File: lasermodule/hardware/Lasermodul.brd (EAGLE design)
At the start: 89 parts, among them IC1 MEGA8-AI

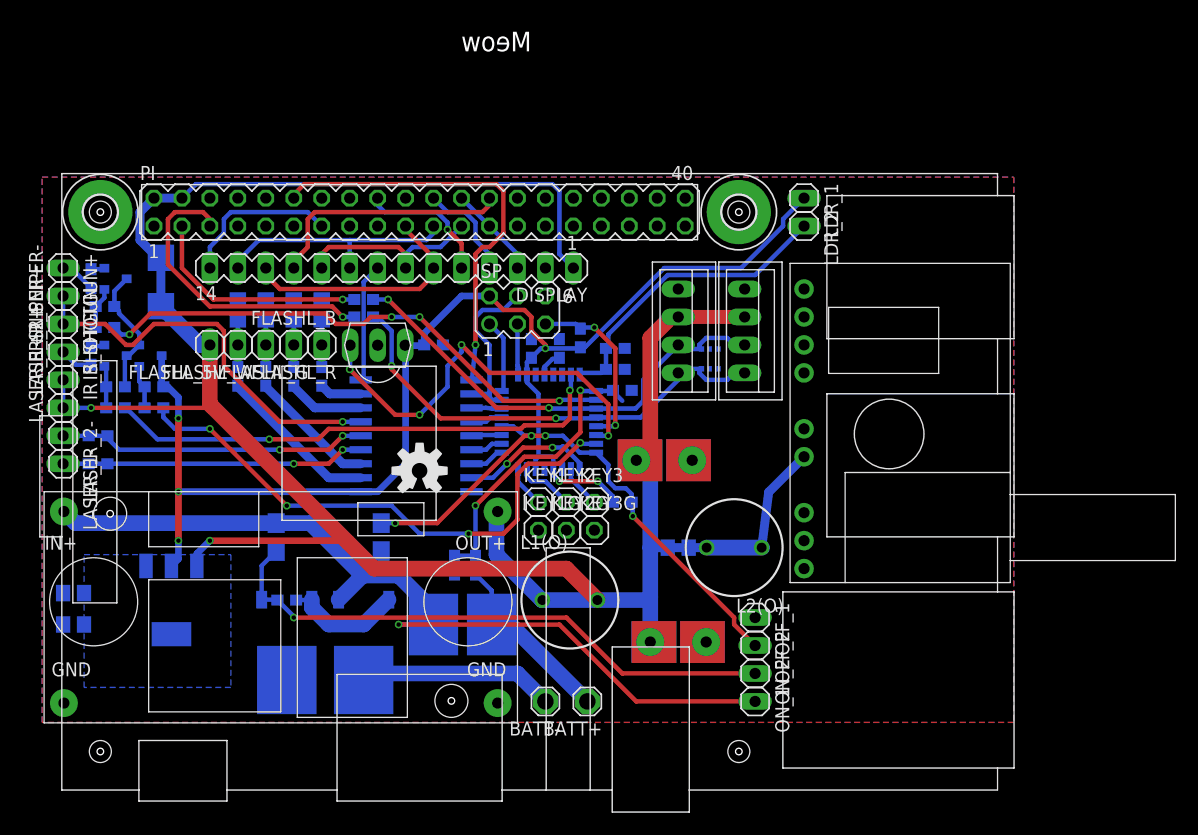
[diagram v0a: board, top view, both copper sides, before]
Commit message: routing
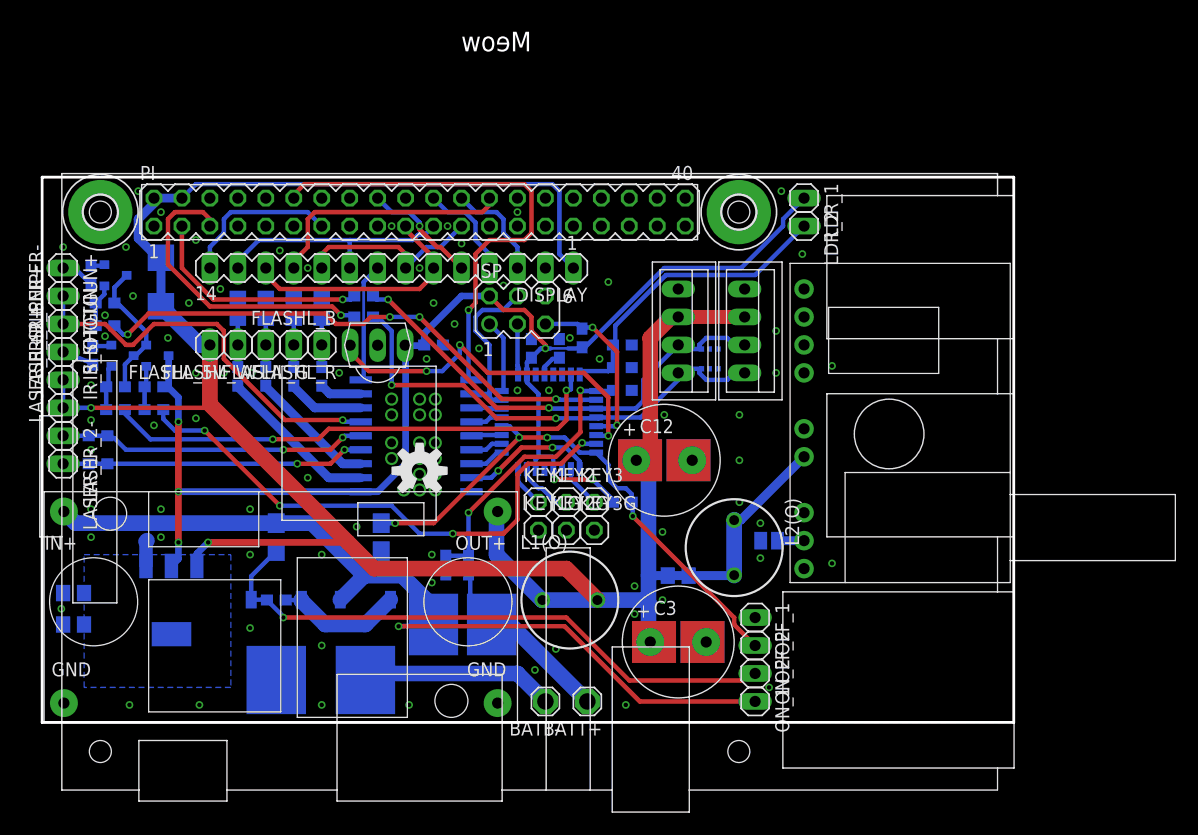
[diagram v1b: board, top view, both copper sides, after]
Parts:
- added SJ1: (no value), jumper:SJ
- moved R3(O) 2.54 mm to (57.8, 13.3)
- moved ON 0.95 mm to (21.3, 6.35)
- moved R9 0.95 mm to (21.3, 11.1)
- moved R5 0.79 mm to (36.7, 14.3)
- moved R16 0.71 mm to (52.7, 34.3)
- moved C4 0.65 mm to (52.7, 32.2)
- moved P-FET1 0.63 mm to (10.5, 33.3)
- moved P-FET2 0.63 mm to (7.30, 33.3)
- moved R4 0.63 mm to (38.7, 14.3)
- moved P-FET3 0.32 mm to (6.67, 40.6)
- moved R23 0.32 mm to (5.71, 38.1)
- moved R24 0.32 mm to (4.45, 40.6)
- moved R6 0.32 mm to (29.2, 38.7)
- moved R22 0.16 mm to (5.71, 36.0)
- moved R21 0.16 mm to (4.60, 33.3)
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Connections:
- net +5V: now also C12.+, C3.+; no longer C12.+A, C12.+B, C12.+C, C3.+A, C3.+B, C3.+C
- net AMP_IN_AGND: now also SJ1.2
- net GND: now also C12.-, C3.-, SJ1.1; no longer C12.-A, C12.-B, C12.-C, C3.-A, C3.-B, C3.-C
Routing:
- net I_BACKLIGHT: track 38.6 -> 44.1 mm
- net RX: track 37.7 -> 32.9 mm, vias 4 -> 3
- net N$45: track 1.63 -> 4.15 mm
- net AMP_IN_AGND: track 0.00 -> 2.41 mm
- net GND: track 0.00 -> 2.34 mm, vias 0 -> 92
- net ONOFF_2: track 52.7 -> 54.6 mm
- net LCD_DC: track 12.3 -> 10.6 mm
- net ONOFF: track 50.5 -> 49.4 mm
- net LCD_CS: track 8.45 -> 9.57 mm
- net EASTEREGG_NET: track 11.9 -> 12.8 mm
- net +3V3: track 122.5 -> 123.4 mm
- net N$46: track 9.63 -> 8.73 mm
- net BATT+_ADC: track 27.3 -> 26.5 mm
- net SCL_BUS: track 43.5 -> 44.3 mm
- net LCD_SCK: track 18.1 -> 17.3 mm
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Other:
- board outline added: 88.3 x 49.5 mm
